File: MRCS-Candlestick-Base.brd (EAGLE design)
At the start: 69.8 x 68.8 mm, 11 parts, among them CON1 Speaker

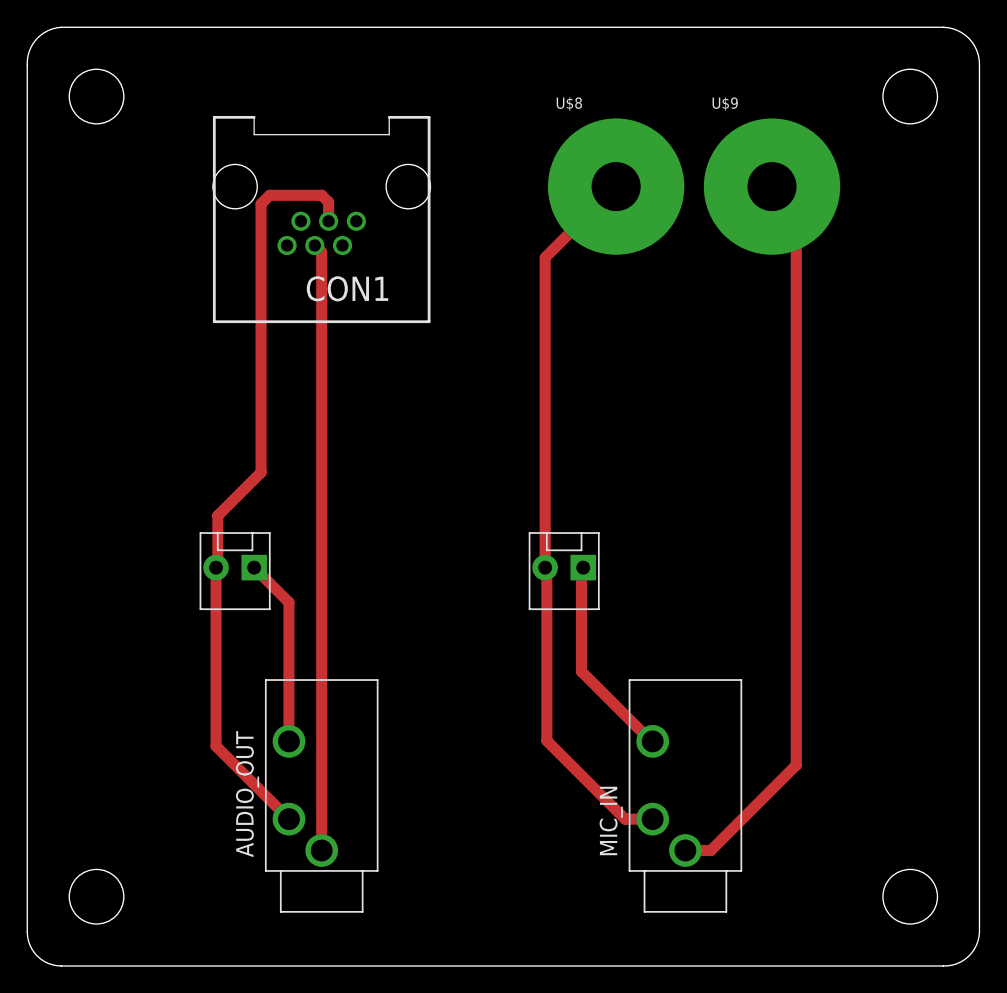
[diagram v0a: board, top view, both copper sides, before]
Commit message: panelized
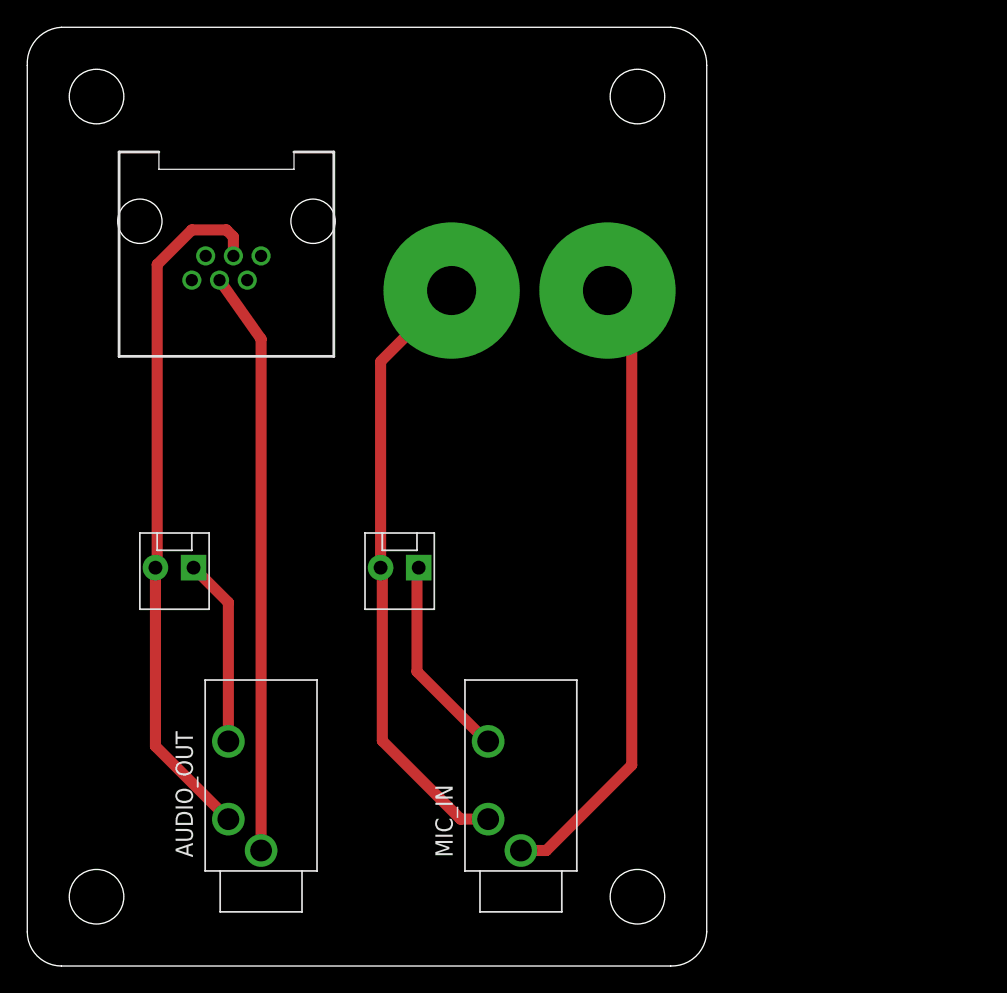
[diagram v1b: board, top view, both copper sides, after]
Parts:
- BOARD1: value BOARD69X70 -> BOARD69X50; device SPCoast:BOARD-DINRAIL-2.7IN-7CM -> SPCoast:BOARD-DINRAIL-2.7IN-5CM
- U$5: device MRCSLogoTop:MRCSLOGOTOP -> SPCoast:MRCSLOGOTOP
- U$6: device MRCSLogoBtm:MRCSLOGOBTM -> SPCoast:MRCSLOGOBTM
- moved U$8 14.3 mm to (31.1, 49.5)
- moved U$9 14.3 mm to (42.5, 49.5)
- moved U$5 14.0 mm to (4.06, 37.8)
- moved U$6 14.0 mm to (4.06, 37.8)
- moved U$7 12.1 mm to (48.6, 33.3)
- moved JP2 12.1 mm to (28.6, 29.2)
- moved MIC_IN 12.1 mm to (36.2, 14.0)
- moved CON1 7.43 mm to (14.6, 54.6)
- moved JP1 4.45 mm to (12.1, 29.2)
- moved AUDIO_OUT 4.45 mm to (17.1, 14.0)
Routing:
- net N$5: track 53.0 -> 45.4 mm
- net N$4: track 53.9 -> 46.3 mm
- net N$1: track 55.5 -> 51.2 mm
- net N$2: track 44.6 -> 42.8 mm
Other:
- board size 69.8 x 68.8 mm -> 49.8 x 68.8 mm
- board text removed: "CON1"
- board text removed: "U$8"
- board text removed: "U$9"
